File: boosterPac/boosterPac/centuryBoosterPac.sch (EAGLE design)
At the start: 37 parts, among them IC1 317T, J1 22-05-7028-02, J2 22-05-7028-02, Q1 BSS123

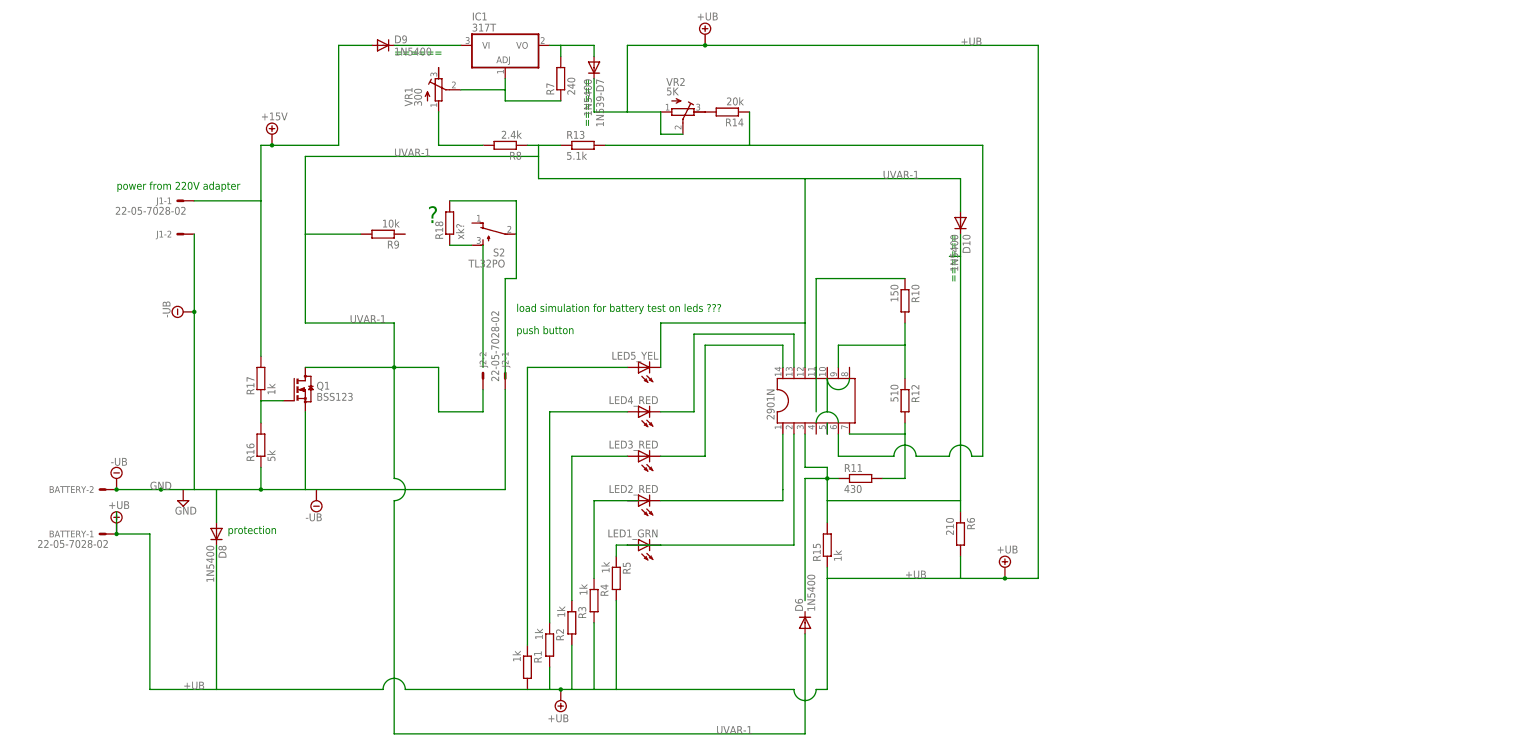
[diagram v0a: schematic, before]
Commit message: reg save
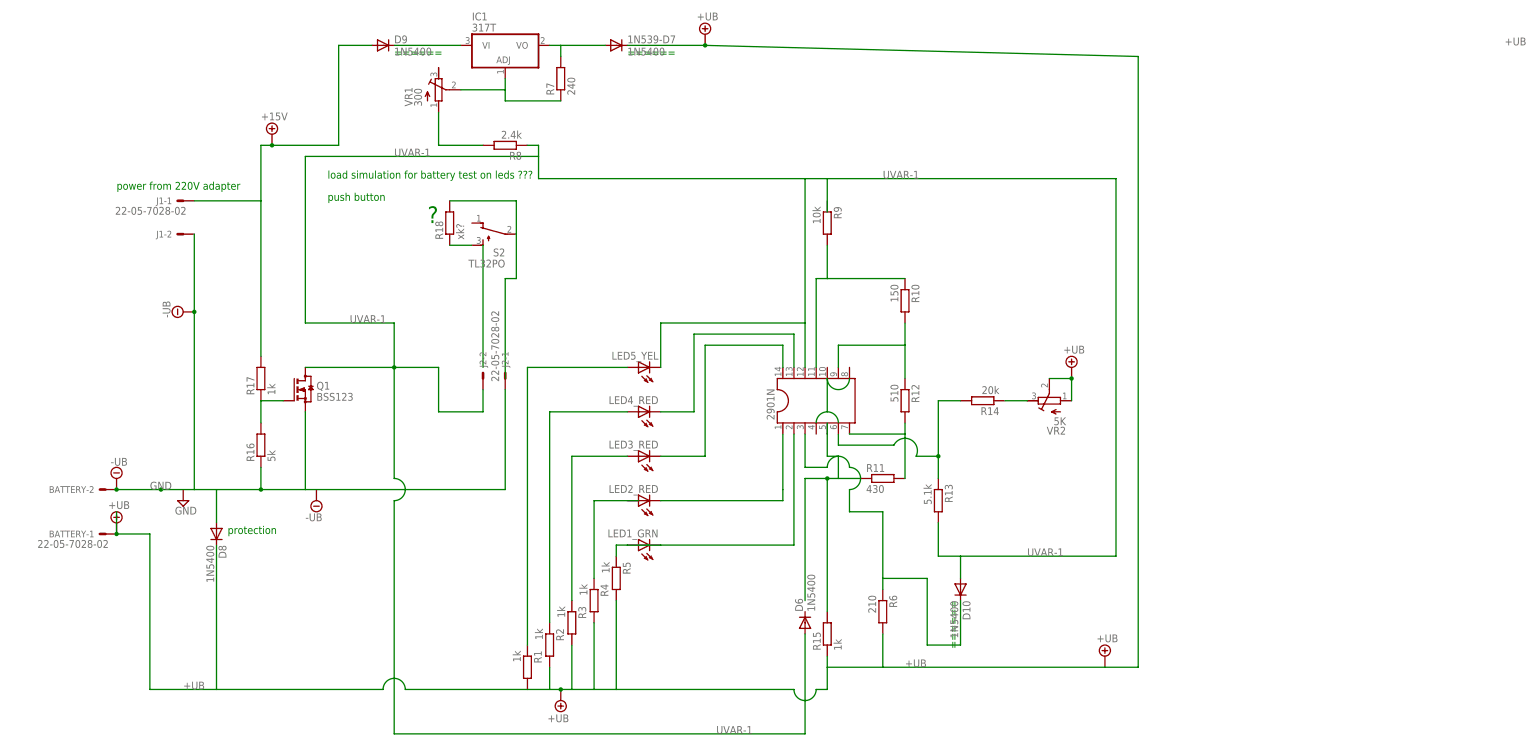
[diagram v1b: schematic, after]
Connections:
- net N$27 renamed N$V12
- net N$12: now also R9.2
- net N$14: now also R11.1, R15.2
- net N$19: now also R13.1, R14.2; no longer R13.2, R14.1
- net N$8: now also R14.1; no longer R14.2
- net N$9: no longer R11.1, R15.2
- net UVAR-1: now also R13.2; no longer R13.1, R9.2
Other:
- moved on the sheet: 1N539-D7, D10, R11, R13, R14, R15, R6, R9, VR2

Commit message: reg save
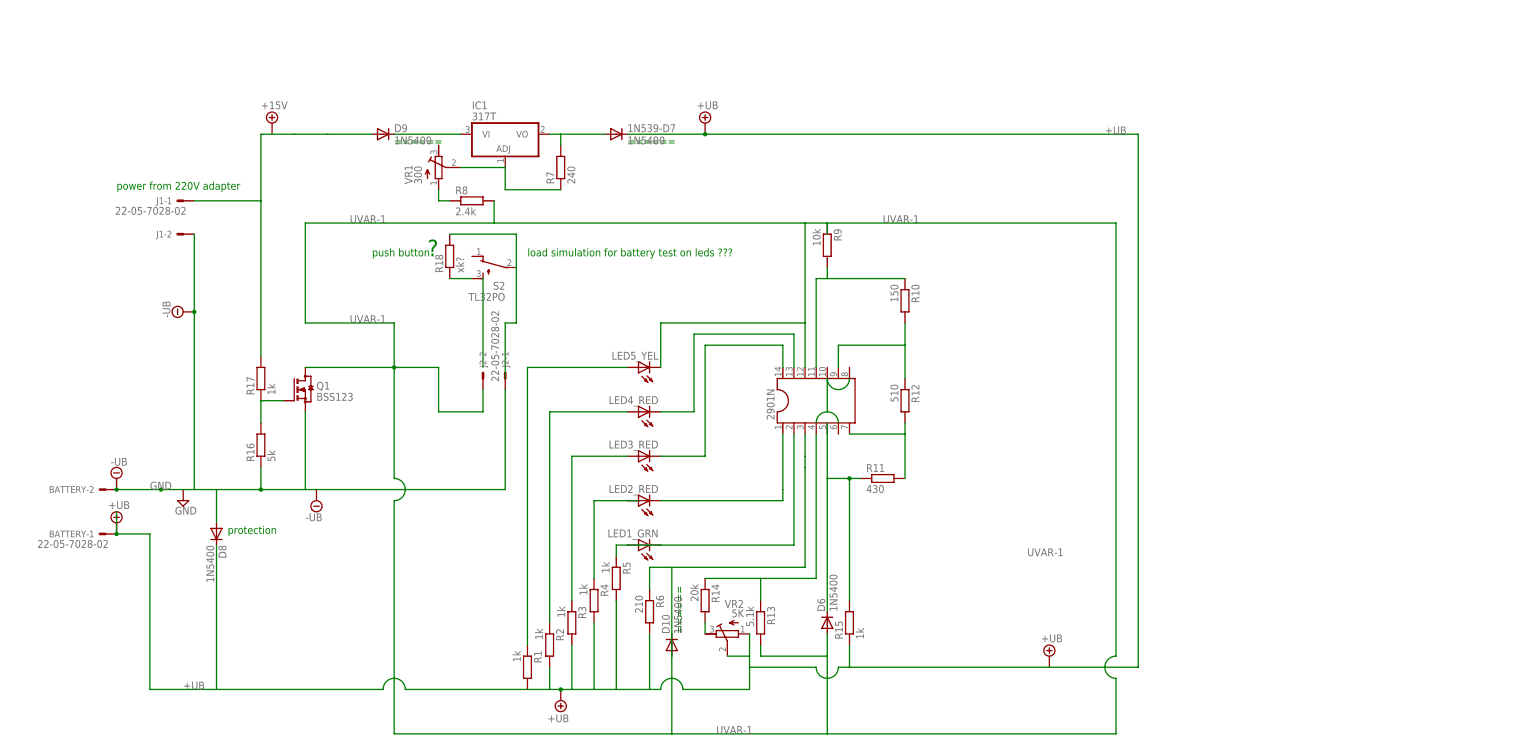
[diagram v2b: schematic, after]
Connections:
- removed net +15V: J1-1.S, R17.2
- removed net N$19: 2901N.6, R13.1, R14.2
- new net N$27: 2901N.3, R6.1
- new net N$30: 2901N.5
- new net N$31: D9.A, J1-1.S, R17.2
- net N$14: now also D6.C; no longer 2901N.5
- net N$29: now also D9.C
- net N$3: now also R8.1; no longer R8.2
- net N$8: now also R14.2; no longer R14.1
- net N$9: now also 2901N.4, R13.1, R14.1; no longer 2901N.3, D10.C, R6.1
- net UVAR-1: now also D10.C, R8.2; no longer R8.1
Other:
- moved on the sheet: 1N539-D7, D10, D6, D9, IC1, R13, R14, R15, R18, R6, R7, R8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
